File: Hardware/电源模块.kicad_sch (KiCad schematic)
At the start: 28 parts, among them J3 Barrel_Jack_Switch, U2 MP2225GJ, U3 AMS1117-1.8, U4 AMS1117-2.5, U5 AMS1117-3.3

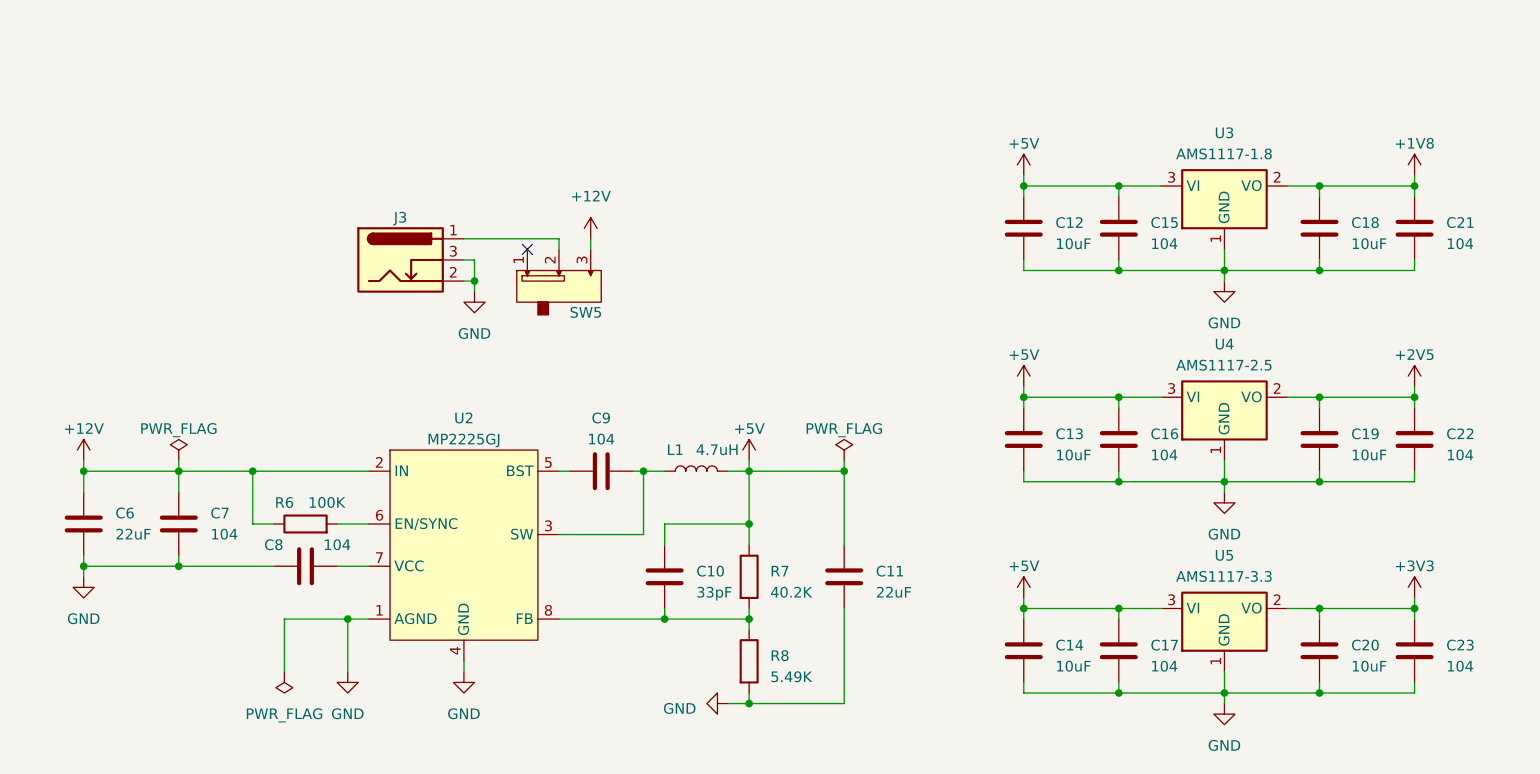
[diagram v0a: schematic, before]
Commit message: nm
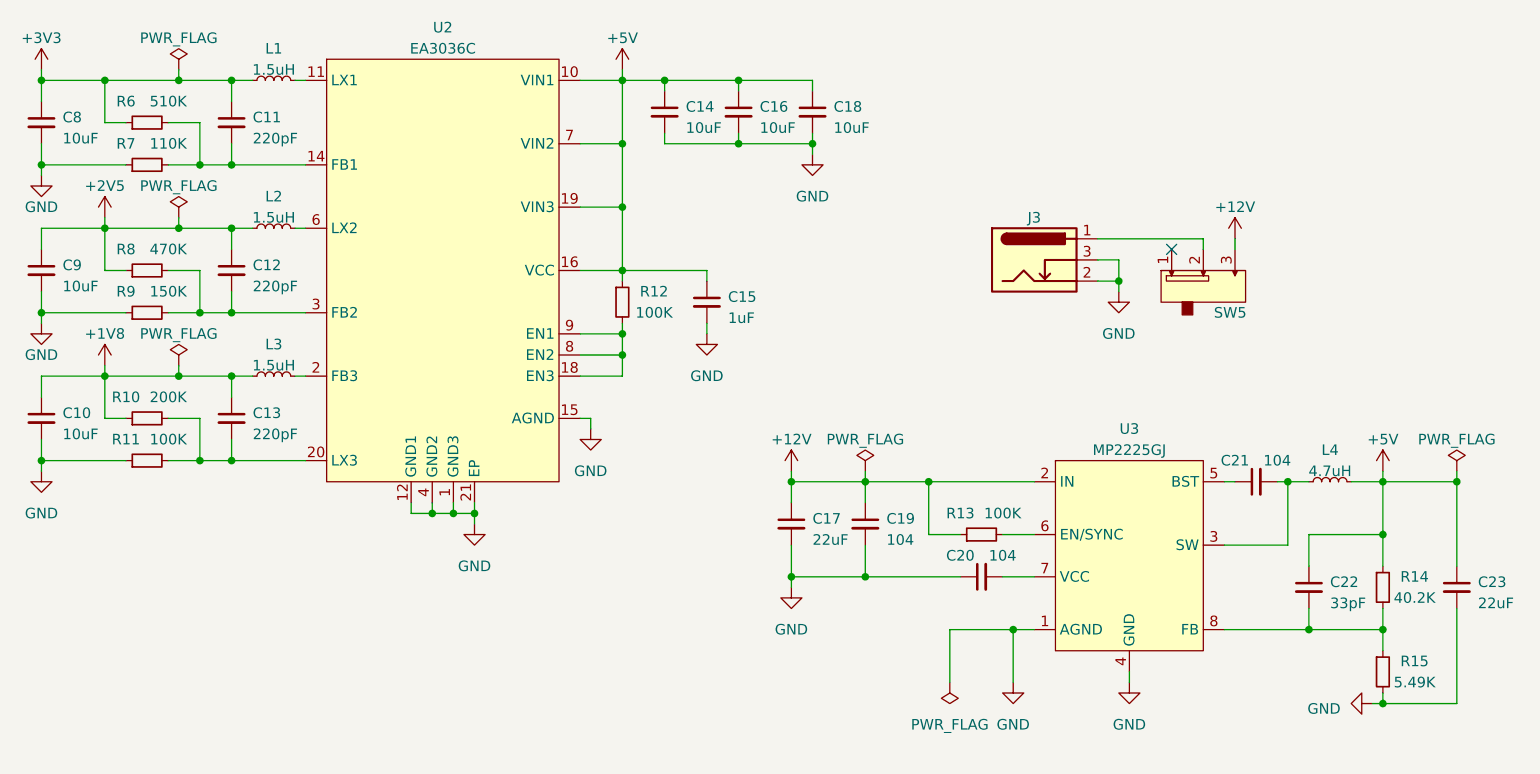
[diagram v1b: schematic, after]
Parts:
- removed C10: 33pF, Capacitor_SMD:C_0402_1005Metric, symbol Device:C
- removed C11: 22uF, Capacitor_SMD:C_1206_3216Metric, symbol Device:C
- removed C12, C13, C14, C18, C19, C20: 10uF, Capacitor_SMD:C_0603_1608Metric, symbol Device:C
- removed C15, C16, C17, C21, C22, C23, C7, C8, C9: 104, Capacitor_SMD:C_0402_1005Metric, symbol Device:C
- removed C6: 22uF, Capacitor_SMD:C_1210_3225Metric, symbol Device:C
- removed L1: 4.7uH, Inductor_SMD:L_Chilisin_BMRx00060630, symbol Device:L
- removed R6: 100K, Resistor_SMD:R_0402_1005Metric, symbol Device:R
- removed R7: 40.2K, Resistor_SMD:R_0402_1005Metric, symbol Device:R
- removed R8: 5.49K, Resistor_SMD:R_0402_1005Metric, symbol Device:R
- removed U3: AMS1117-1.8, Package_TO_SOT_SMD:SOT-223-3_TabPin2, symbol Regulator_Linear:AMS1117-1.8
- removed U4: AMS1117-2.5, Package_TO_SOT_SMD:SOT-223-3_TabPin2, symbol Regulator_Linear:AMS1117-2.5
- removed U5: AMS1117-3.3, Package_TO_SOT_SMD:SOT-223-3_TabPin2, symbol Regulator_Linear:AMS1117-3.3
- added C10, C14, C16, C18, C8, C9: 10uF, Capacitor_SMD:C_0402_1005Metric, symbol Device:C_Small
- added C11, C12, C13: 220pF, Capacitor_SMD:C_0402_1005Metric, symbol Device:C_Small
- added C15: 1uF, Capacitor_SMD:C_0402_1005Metric, symbol Device:C_Small
- added C17, C23: 22uF, Capacitor_SMD:C_0805_2012Metric, symbol Device:C_Small
- added C19, C20, C21: 104, Capacitor_SMD:C_0402_1005Metric, symbol Device:C_Small
- added C22: 33pF, Capacitor_SMD:C_0402_1005Metric, symbol Device:C_Small
- added L1, L2, L3: 1.5uH, Inductor_SMD:L_Chilisin_BMRA00050520, symbol Device:L_Small
- added L4: 4.7uH, Inductor_SMD:L_Chilisin_BMRA00050520, symbol Device:L_Small
- added R10: 200K, Resistor_SMD:R_0402_1005Metric, symbol Device:R_Small
- added R11, R12, R13: 100K, Resistor_SMD:R_0402_1005Metric, symbol Device:R_Small
- added R14: 40.2K, Resistor_SMD:R_0402_1005Metric, symbol Device:R_Small
- added R15: 5.49K, Resistor_SMD:R_0402_1005Metric, symbol Device:R_Small
- added R6: 510K, Resistor_SMD:R_0402_1005Metric, symbol Device:R_Small
- added R7: 110K, Resistor_SMD:R_0402_1005Metric, symbol Device:R_Small
- added R8: 470K, Resistor_SMD:R_0402_1005Metric, symbol Device:R_Small
- added R9: 150K, Resistor_SMD:R_0402_1005Metric, symbol Device:R_Small
- added U2: EA3036C, Package_DFN_QFN:QFN-20-1EP_3x3mm_P0.4mm_EP1.65x1.65mm, symbol Power_Management:EA3036C
- renumbered U2 to U3
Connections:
- net +12V: now also C17.1, C19.1, R13.1
- net +1V8: now also C10.1, C13.1, L3.1, R10.1
- net +2V5: now also C12.1, C9.1, L2.1, R8.1
- net +3V3: now also C11.1, C8.1, L1.1, R6.1
- net +5V: now also C14.1, C15.1, C16.1, C18.1, C22.1, C23.1, L4.2, R12.1, R14.1, U2.10 (VIN1), U2.16 (VCC), U2.19 (VIN3), U2.7 (VIN2)
- net GND: now also C10.2, C14.2, C15.2, C16.2, C17.2, C18.2, C19.2, C20.1, C23.2, C8.2, C9.2, R11.1, R15.2, R7.1, R9.1, U2.1 (GND3), U2.12 (GND1), U2.13 (GND1), U2.15 (AGND), U2.17 (AGND), U2.21 (EP), U2.4 (GND2), U2.5 (GND2)
- net at U3.8 (FB): now also C22.2, R14.2, R15.1
- net at U3.7 (VCC): now also C20.2
- net at U3.3 (SW): now also C21.2, L4.1
- net at U3.6 (EN/SYNC): now also R13.2
- net at U3.5 (BST): now also C21.1
- new net: L3.2, U2.2 (FB3)
- new net: L1.2, U2.11 (LX1)
- new net: C12.2, R8.2, R9.2, U2.3 (FB2)
- new net: C11.2, R6.2, R7.2, U2.14 (FB1)
- new net: R12.2, U2.18 (EN3), U2.8 (EN2), U2.9 (EN1)
- new net: C13.2, R10.2, R11.2, U2.20 (LX3)
- new net: L2.2, U2.6 (LX2)
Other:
- moved on the sheet: J3, SW5, U3

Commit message: nm
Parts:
- J3: footprint Connector_BarrelJack:BarrelJack_CLIFF_FC681465S_SMT_Horizontal -> Connector_BarrelJack:BarrelJack_XKB_DC-044A-2.5A-2.5
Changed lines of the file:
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@@
       (effects (font (size 1.27 1.27)) hide)
     )
-    (property "Footprint" "Connector_BarrelJack:BarrelJack_CLIFF_FC681465S_SMT_Horizontal" (at 137.16 44.196 0)
+    (property "Footprint" "Connector_BarrelJack:BarrelJack_XKB_DC-044A-2.5A-2.5" (at 137.16 44.196 0)
       (effects (font (size 1.27 1.27)) hide)
     )
